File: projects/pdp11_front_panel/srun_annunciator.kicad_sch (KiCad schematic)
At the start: 11 parts

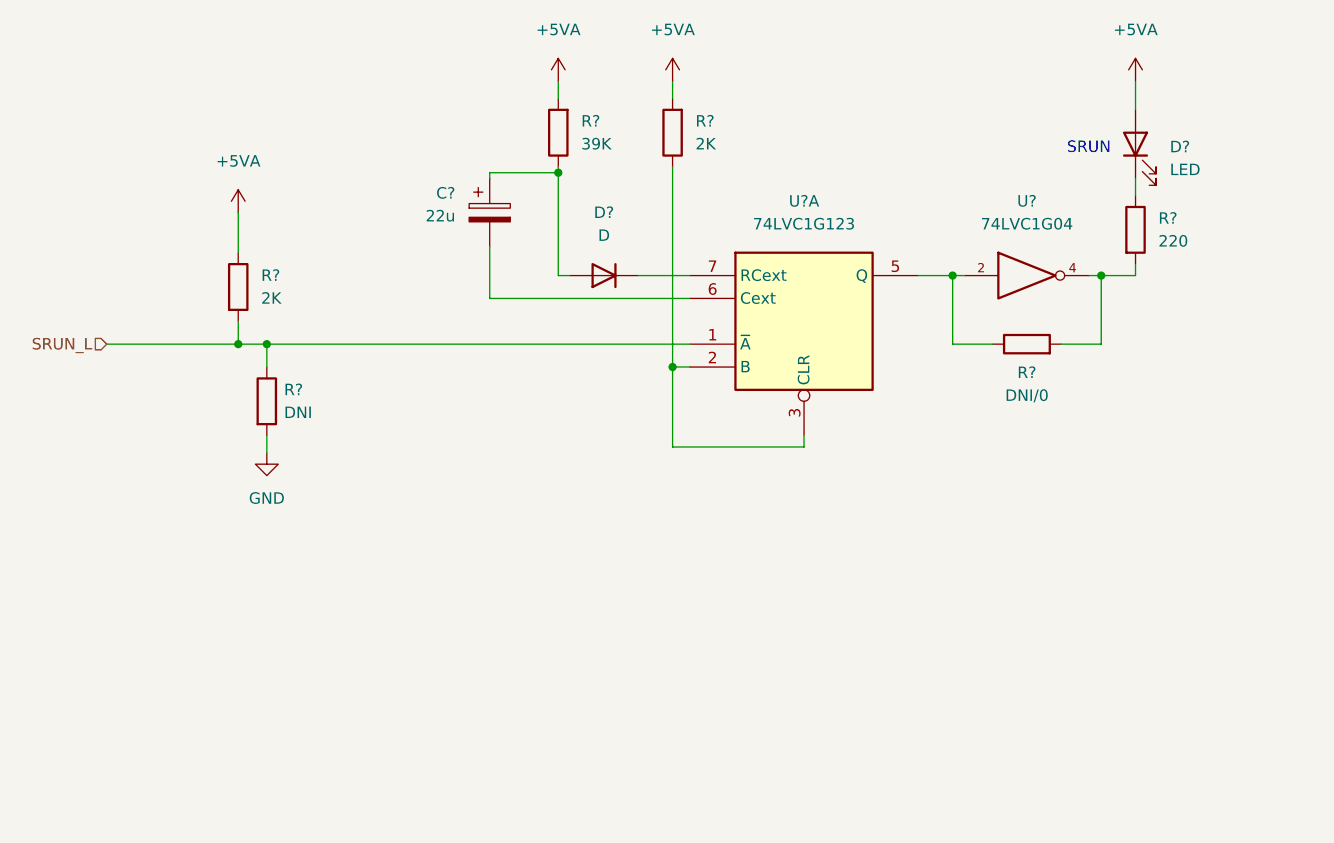
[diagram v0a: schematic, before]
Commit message: .
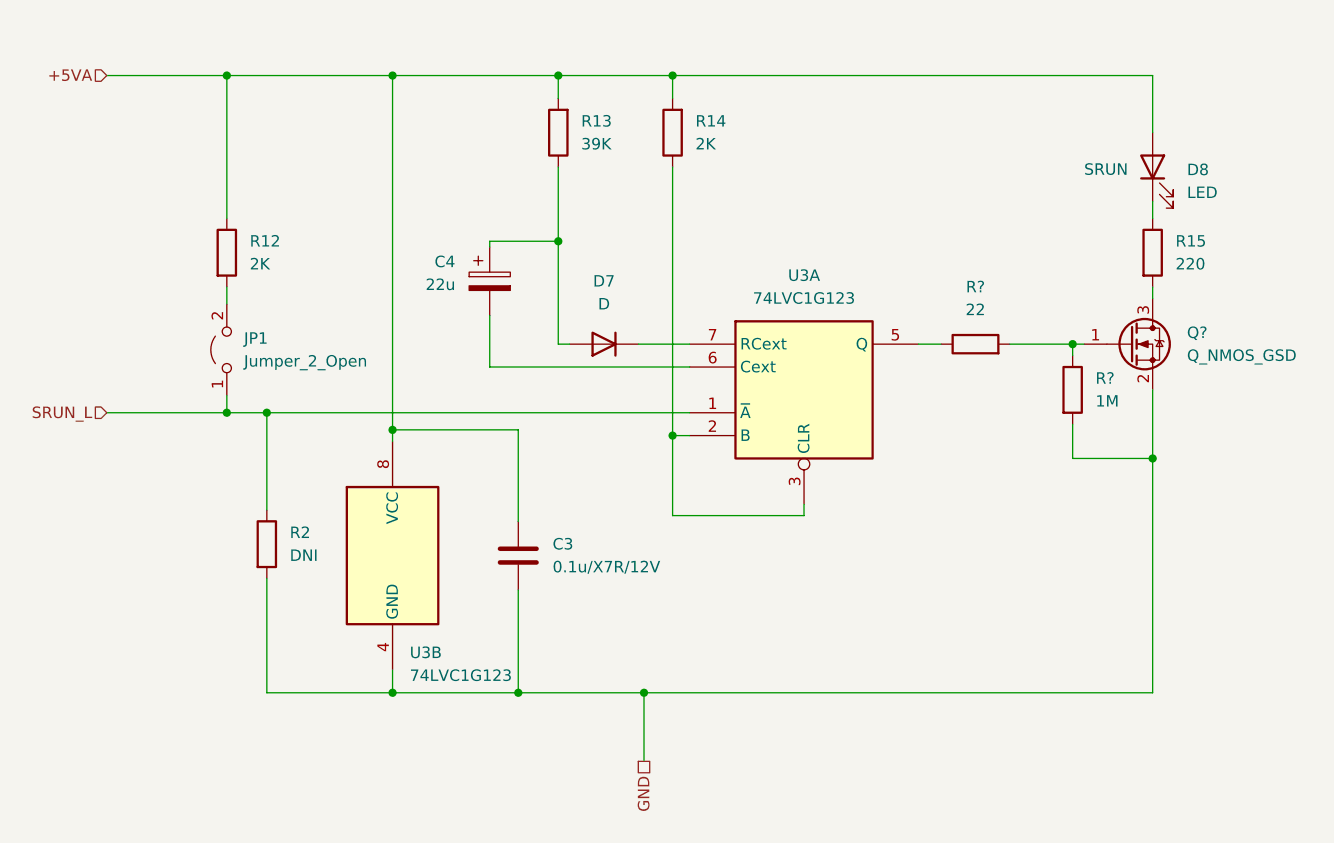
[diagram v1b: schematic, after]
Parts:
- removed R?: DNI/0, symbol Device:R
- removed R?: DNI, symbol Device:R
- removed U?: 74LVC1G04, symbol 74xGxx:74LVC1G04
- added C3: 0.1u/X7R/12V, symbol Device:C
- added JP1: Jumper_2_Open, symbol Jumper:Jumper_2_Open
- added Q?: Q_NMOS_GSD, symbol Device:Q_NMOS_GSD
- added R2: DNI, symbol Device:R
- added R?: 22, symbol Device:R
- added R?: 1M, symbol Device:R
- added unit 2 of U3
- gave numbers to parts that had none: 8
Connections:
- net +5VA: now also C3.1, U3.8 (VCC)
- net GND: now also C3.2, Q?.2 (S), R2.2, R?.2, U3.4 (GND)
- net SRUN_L: now also JP1.1 (A), R2.1; no longer R12.2
- net at U3.5 (Q): now also R?.1
- net at R15.2: now also Q?.3 (D)
- new net: JP1.2 (B), R12.2
- new net: Q?.1 (G), R?.1, R?.2
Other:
- moved on the sheet: C4, D7, D8, R12, R15, U3A

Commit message: wip
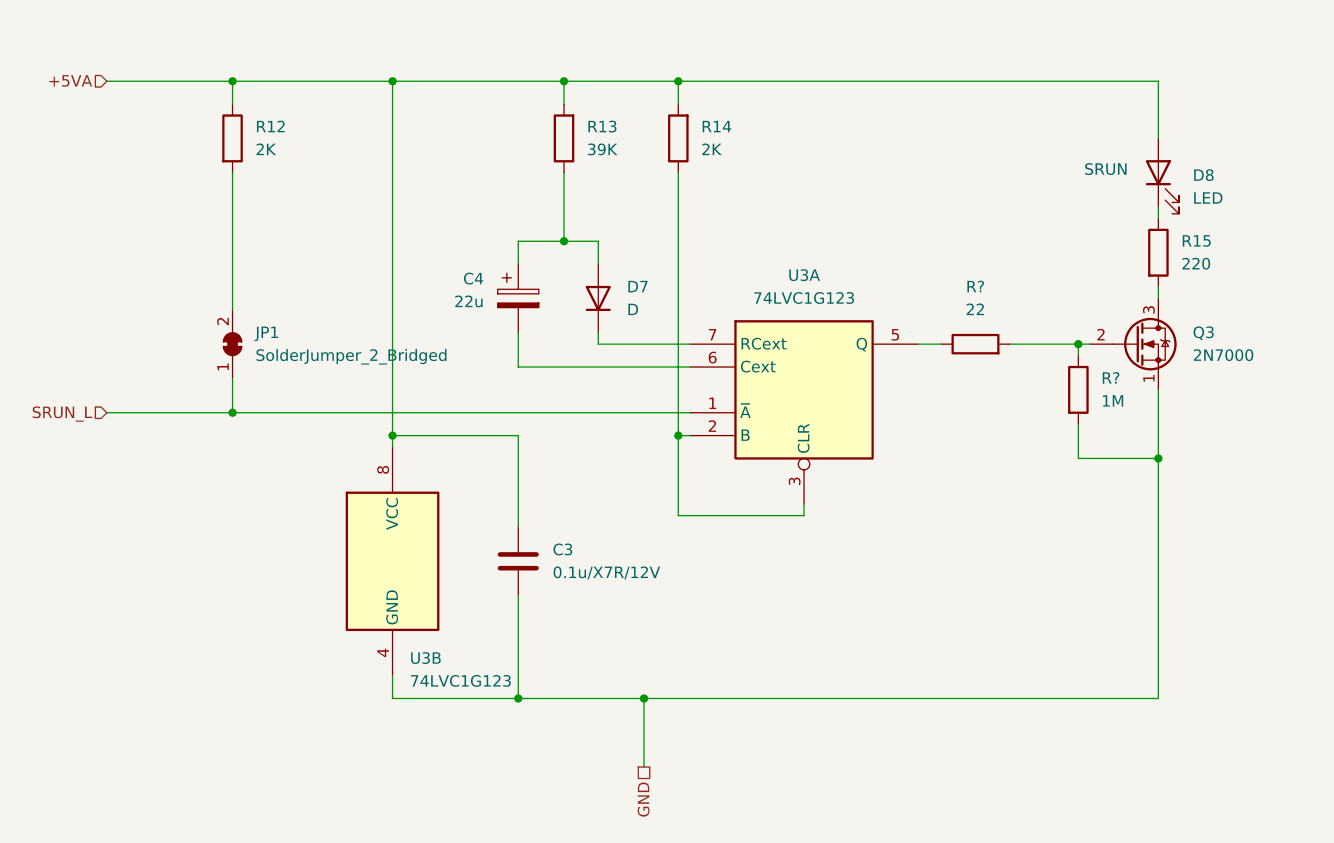
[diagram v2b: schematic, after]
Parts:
- removed JP1: Jumper_2_Open, symbol Jumper:Jumper_2_Open
- removed Q?: Q_NMOS_GSD, symbol Device:Q_NMOS_GSD
- removed R2: DNI, symbol Device:R
- added JP1: SolderJumper_2_Bridged, symbol Jumper:SolderJumper_2_Bridged
- added Q3: 2N7000, Package_TO_SOT_THT:TO-92_Inline, symbol Transistor_FET:2N7000
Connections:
- net GND: now also Q3.1 (S)
- net SRUN_L: now also JP1.1 (A)
- net at R12.2: now also JP1.2 (B)
- net at R?.1, R?.2: now also Q3.2 (G)
- net at R15.2: now also Q3.3 (D)
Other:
- moved on the sheet: C3, C4, D7, D8, R12, R13, R14, R15, R?, U3B
